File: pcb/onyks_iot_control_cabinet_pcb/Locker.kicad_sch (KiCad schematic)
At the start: 9 parts, among them J2 Screw_Terminal_01x02, J7 Conn_01x02_Socket, Q3 SQ4050EY-T1_GE3, Q4 SQ4050EY-T1_GE3, SW1 SW_Push

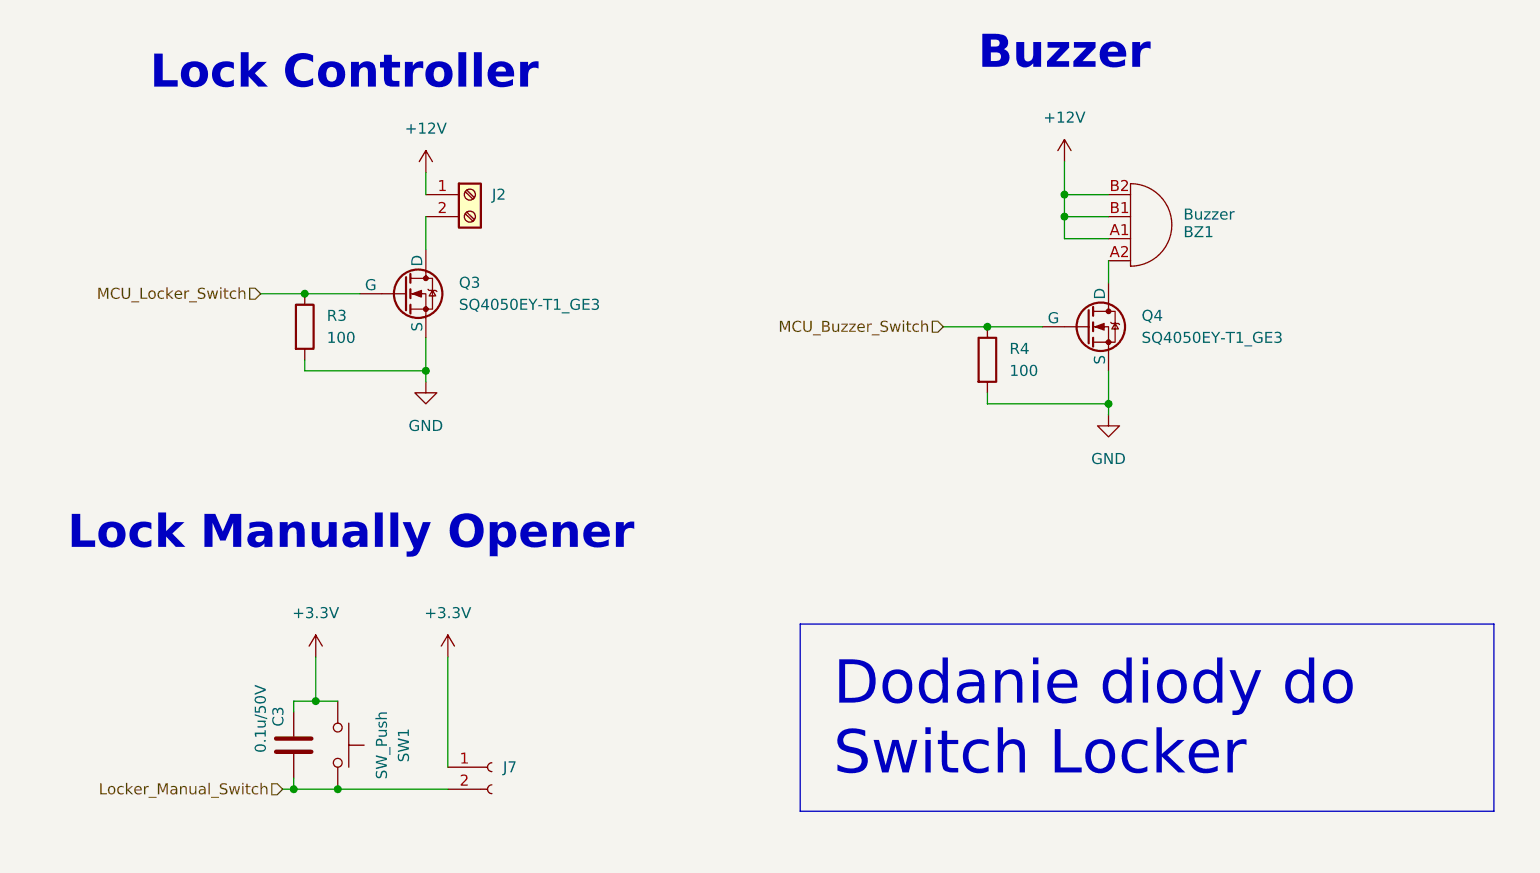
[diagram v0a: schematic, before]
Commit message: Quick Fixes
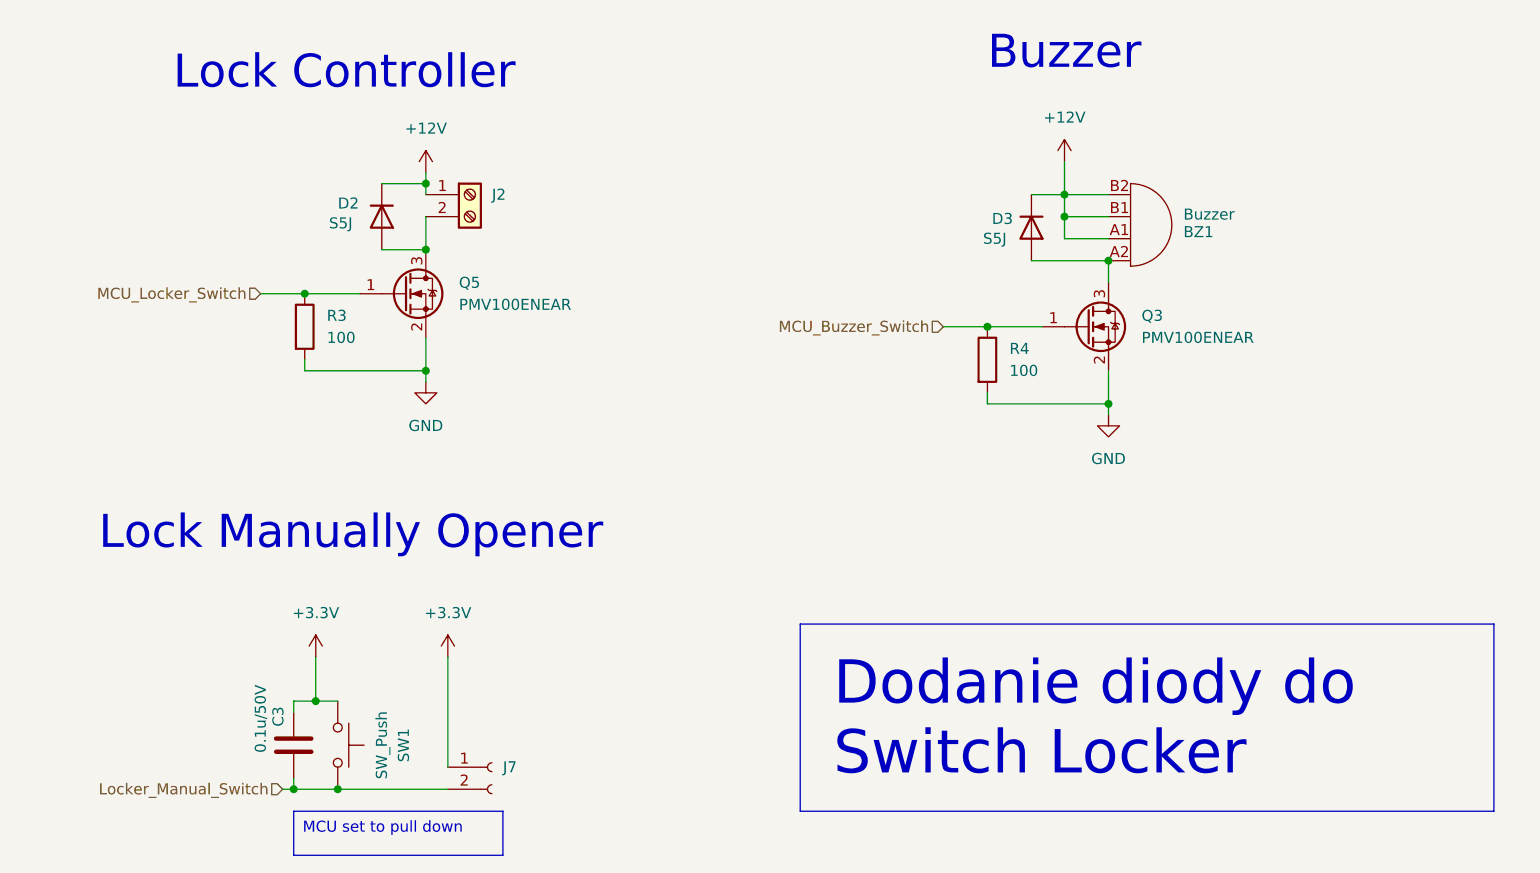
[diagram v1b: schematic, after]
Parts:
- removed Q3, Q4: SQ4050EY-T1_GE3, ourFootprints:SOIC127P600X175-8N, symbol Simulation_SPICE:NMOS
- added D2, D3: S5J, Diode_SMD:D_SMC, symbol Diode:STTH212S
- added Q3, Q5: PMV100ENEAR, Package_TO_SOT_SMD:SOT-23, symbol Transistor_FET:2N7002
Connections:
- net +12V: now also D2.1 (K), D3.1 (K)
- net GND: now also Q3.2 (S), Q5.2 (S)
- net MCU_Buzzer_Switch: now also Q3.1 (G)
- net MCU_Locker_Switch: now also Q5.1 (G)
- net at J2.2 (Pin_2): now also D2.2 (A), Q5.3 (D)
- net at BZ1.A2 (-_2): now also D3.2 (A), Q3.3 (D)
